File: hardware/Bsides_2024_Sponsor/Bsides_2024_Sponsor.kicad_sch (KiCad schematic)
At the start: 42 parts, among them J1 OLED, J2 Battery, J3 Battery, J5 Add_On, P1 USB_C_Plug_USB2.0, Q1 DMG3415U-7, SW1 ON, SW2 RESET, SW3 BOOT, SW4 RESET, SW6 RESET, U1 ESP32-C6-WROOM-1U-N4, U2 AP2112K-3.3

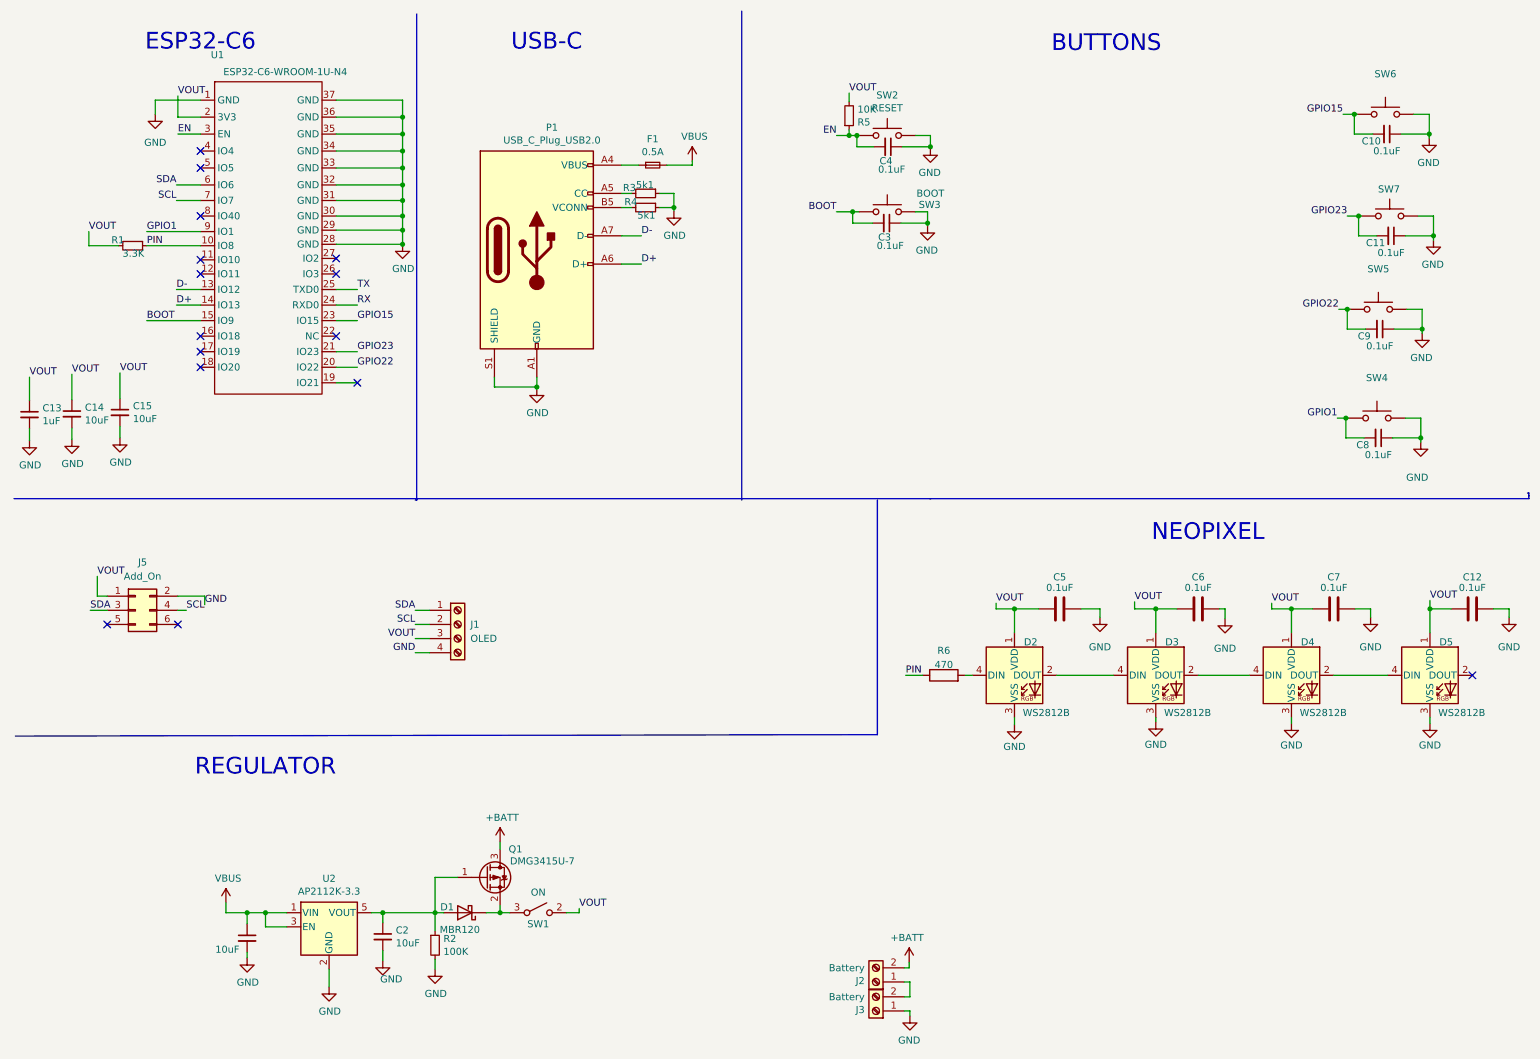
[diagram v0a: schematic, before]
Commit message: feat(Hw):Update_Route_Sponsor
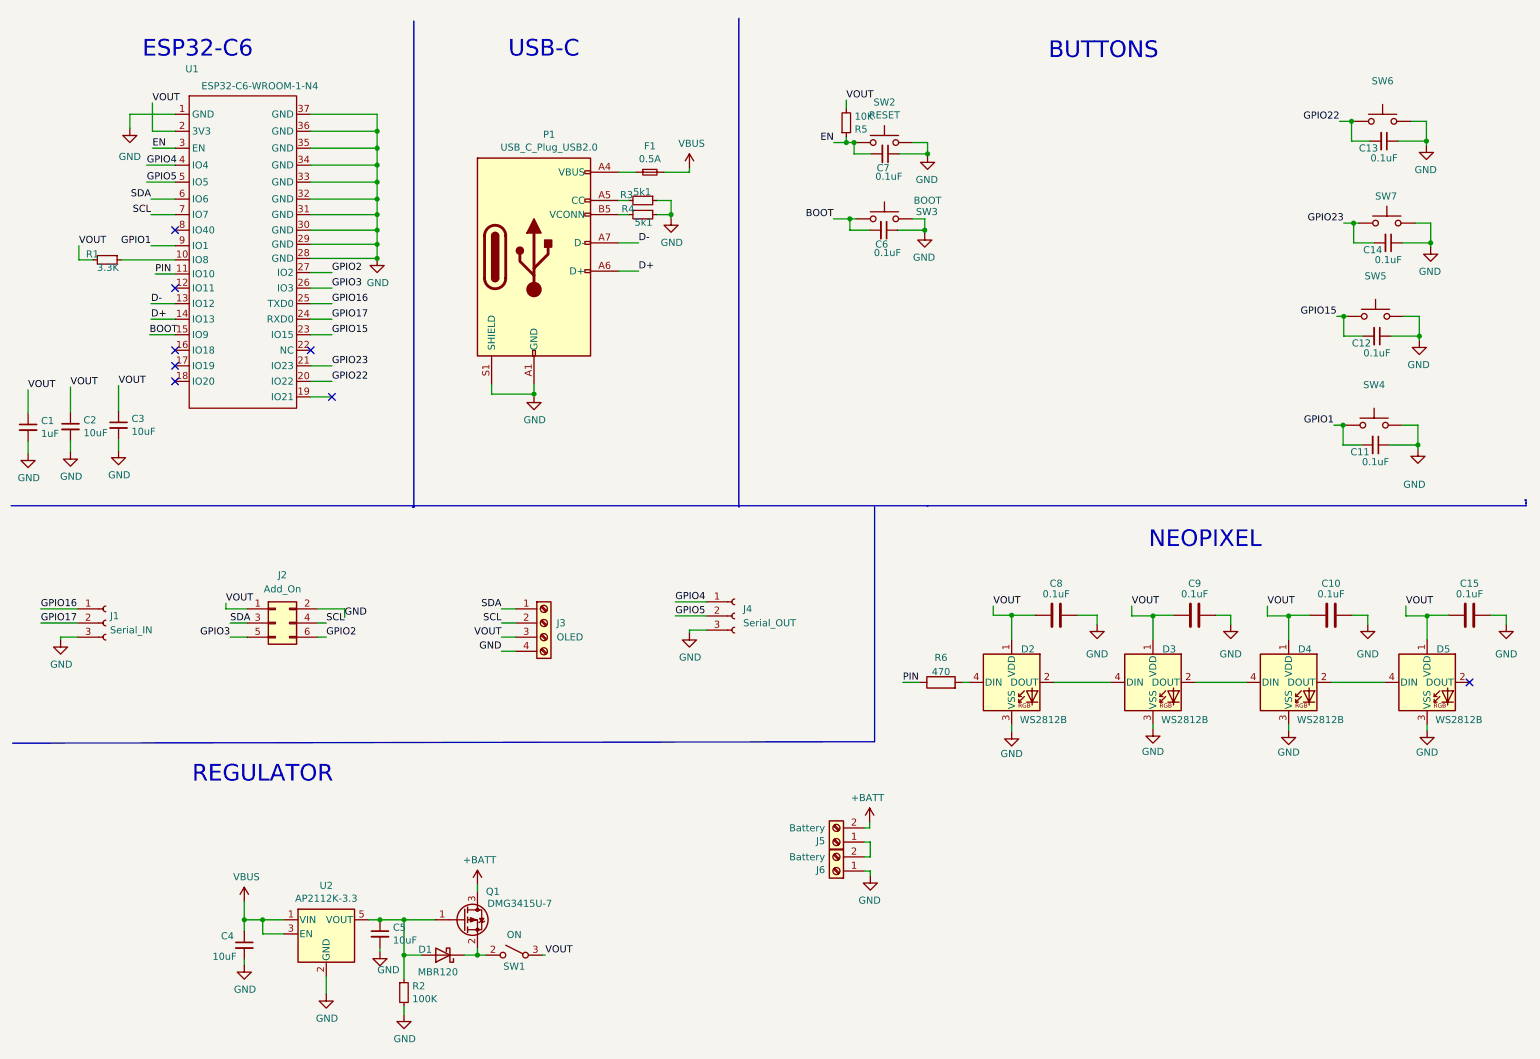
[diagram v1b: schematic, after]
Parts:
- removed C10, C8, C9: 0.1uF, Capacitor_SMD:C_0603_1608Metric, symbol Device:C_Small
- removed C12, C5, C6, C7: 0.1uF, Capacitor_SMD:C_0603_1608Metric, symbol Device:C
- removed C15: 10uF, Capacitor_SMD:C_0603_1608Metric, symbol Device:C_Small
- removed J1: OLED, bsides:Display OLED 128 x32, symbol Connector:Screw_Terminal_01x04
- removed J2, J3: Battery, bsides:BH-AAA-A1aj001, symbol Connector:Screw_Terminal_01x02
- removed J5: Add_On, Connector_PinSocket_2.54mm:PinSocket_2x03_P2.54mm_Vertical, symbol Connector_Generic:Conn_02x03_Odd_Even
- added C10, C15, C8, C9: 0.1uF, Capacitor_SMD:C_0603_1608Metric, symbol Device:C
- added C12, C6, C7: 0.1uF, Capacitor_SMD:C_0603_1608Metric, symbol Device:C_Small
- added C5: 10uF, Capacitor_SMD:C_0603_1608Metric, symbol Device:C_Small
- added J1: Serial_IN, Connector_PinSocket_2.54mm:PinSocket_1x03_P2.54mm_Vertical, symbol Connector:Conn_01x03_Socket
- added J2: Add_On, Connector_PinSocket_2.54mm:PinSocket_2x03_P2.54mm_Vertical, symbol Connector_Generic:Conn_02x03_Odd_Even
- added J3: OLED, bsides:Display OLED 128 x32, symbol Connector:Screw_Terminal_01x04
- added J4: Serial_OUT, Connector_PinHeader_2.54mm:PinHeader_1x03_P2.54mm_Vertical, symbol Connector:Conn_01x03_Socket
- added J5, J6: Battery, bsides:BH-AA-A1AJ020, symbol Connector:Screw_Terminal_01x02
- C1: value 10uF -> 1uF; LCSC# C85713 -> C15849; Proveedor (none) -> Mouser; manf# (none) -> TMK107BJ105KA8T
- C11: LCSC# (none) -> C478888; Proveedor (none) -> Mouser; manf# (none) -> KAM15AR71C104KM
- C13: value 1uF -> 0.1uF; LCSC# C15849 -> C478888; Proveedor (none) -> Mouser; manf# (none) -> KAM15AR71C104KM; provedor LCSC -> (none)
- C14: value 10uF -> 0.1uF; LCSC# C85713 -> C478888; Proveedor (none) -> Mouser; manf# (none) -> KAM15AR71C104KM; provedor LCSC -> (none)
- C2: Proveedor (none) -> Mouser; manf# (none) -> GRM188R61E106KA73J
- C3, C4: value 0.1uF -> 10uF; LCSC# C478888 -> C85713; Proveedor (none) -> Mouser; manf# (none) -> GRM188R61E106KA73J
- D1: Proveedor (none) -> Mouser; manf# MBR120LSF -> MBR120LSFT1G
- D2, D3, D4, D5: manf# WS2812B-Mini -> (none)
- F1: LCSC# - -> (none); Proveedor (none) -> Mouser; manf# MFU0805FF00500P100 -> MFU0805FF00750P100
- P1: Proveedor (none) -> Mouser; manf# TYPE-C-31-M-31 -> USB4105-GF-A
- Q1: Proveedor (none) -> Mouser; manf# DMG3415U-7 -> DMG3415UQ-7
- R1: Proveedor (none) -> Mouser; manf# (none) -> ERJ-3GEYJ332V
- R2: Proveedor LCSC -> Mouser; manf# (none) -> RC0603DR-07100KL
- R3, R4: Proveedor (none) -> Mouser; manf# ERJ3RBD5101V -> AC0603DR-075K1L
- R5: Proveedor (none) -> Mouser; manf# CR-03JL7---10K -> RMC1/16K1002DTP
- R6: Proveedor (none) -> Mouser; manf# RTT03471JTP -> ERJ-3RBD4700V
- SW1, U2: Proveedor (none) -> Mouser
- SW2, SW3, SW5, SW7: Proveedor (none) -> Mouser; manf# (none) -> TL3342F160QG
- SW4, SW6: LCSC# C2886897 -> C318889; Proveedor (none) -> Mouser; manf# (none) -> TL3342F160QG
- U1: value ESP32-C6-WROOM-1U-N4 -> ESP32-C6-WROOM-1-N4; Proveedor (none) -> Mouser; manf# ESP32-C6-WROOM-1U-N4 -> ESP32-C6-WROOM-1-N4
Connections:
- net +BATT: now also J5.2 (Pin_2)
- net BOOT: now also C6.2; no longer C3.2
- net EN: now also C7.2; no longer C4.2
- net GND: now also C13.1, C14.1, C3.2, C4.2, C10.1, C12.1, C15.1, C5.2, C6.1, C7.1, C8.1, C9.1, J1.3 (Pin_3), J2.2 (Pin_2), J3.4 (Pin_4), J4.3 (Pin_3), J6.1 (Pin_1); no longer C13.2, C14.2, C3.1, C4.1
- net GPIO1: now also C11.2
- net GPIO15: now also SW5.2, C12.2; no longer SW6.2
- net GPIO22: now also C13.2, SW6.2; no longer SW5.2
- net GPIO23: now also C14.2; no longer C11.2
- net PIN: now also U1.11 (IO10); no longer R1.1, U1.10 (IO8)
- net SCL: now also J2.4 (Pin_4), J3.2 (Pin_2)
- net SDA: now also J2.3 (Pin_3), J3.1 (Pin_1)
- net VBUS: now also C4.1; no longer C1.1
- net VOUT: now also C1.1, C2.1, C3.1, SW1.3 (A), C10.2, C15.2, C8.2, C9.2, J2.1 (Pin_1), J3.3 (Pin_3); no longer C13.1, C14.1, SW1.2 (B)
- net GPIO3: now reaches U1.26 (IO3)
- net GPIO3: now also J2.5 (Pin_5)
- net GPIO2: now reaches U1.27 (IO2)
- net GPIO2: now also J2.6 (Pin_6)
- net GPIO4: now reaches U1.4 (IO4)
- net GPIO4: now also J4.1 (Pin_1)
- net GPIO5: now reaches U1.5 (IO5)
- net GPIO5: now also J4.2 (Pin_2)
- net at D1.2 (A), Q1.1 (G), R2.1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: now also C5.1; no longer C2.1
- net at D1.1 (K), Q1.2 (S): now also SW1.2 (B); no longer SW1.3 (A)
- net RX renamed GPIO17
- net GPIO17: now also J1.2 (Pin_2)
- net TX renamed GPIO16
- net GPIO16: now also J1.1 (Pin_1)
- new net: R1.1, U1.10 (IO8)
- new net: J5.1 (Pin_1), J6.2 (Pin_2)
- no-connect marks 15 -> 8
